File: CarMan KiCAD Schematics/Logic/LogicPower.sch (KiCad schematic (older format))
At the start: 5 parts, among them U4 PYB20-Q24-S5, U7 LT1763CS8-3.3PBF

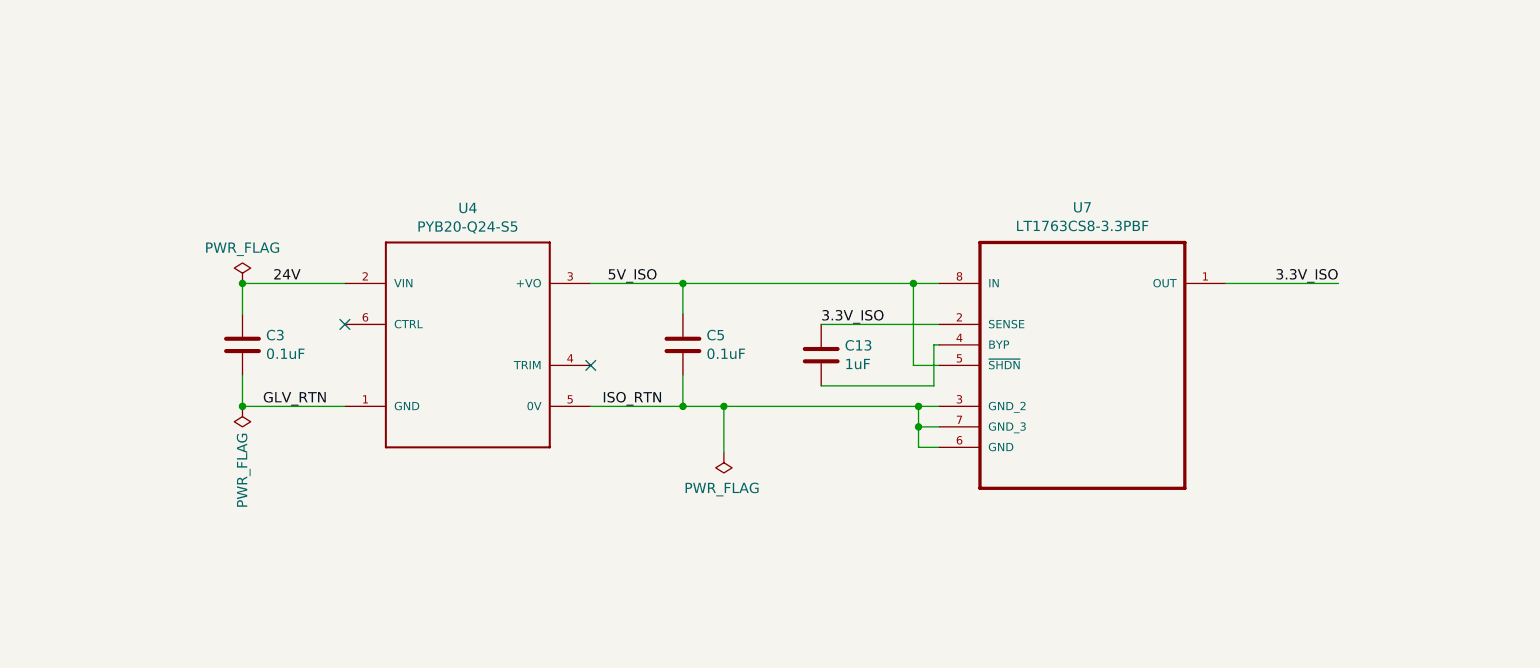
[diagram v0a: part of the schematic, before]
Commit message: Logic Update
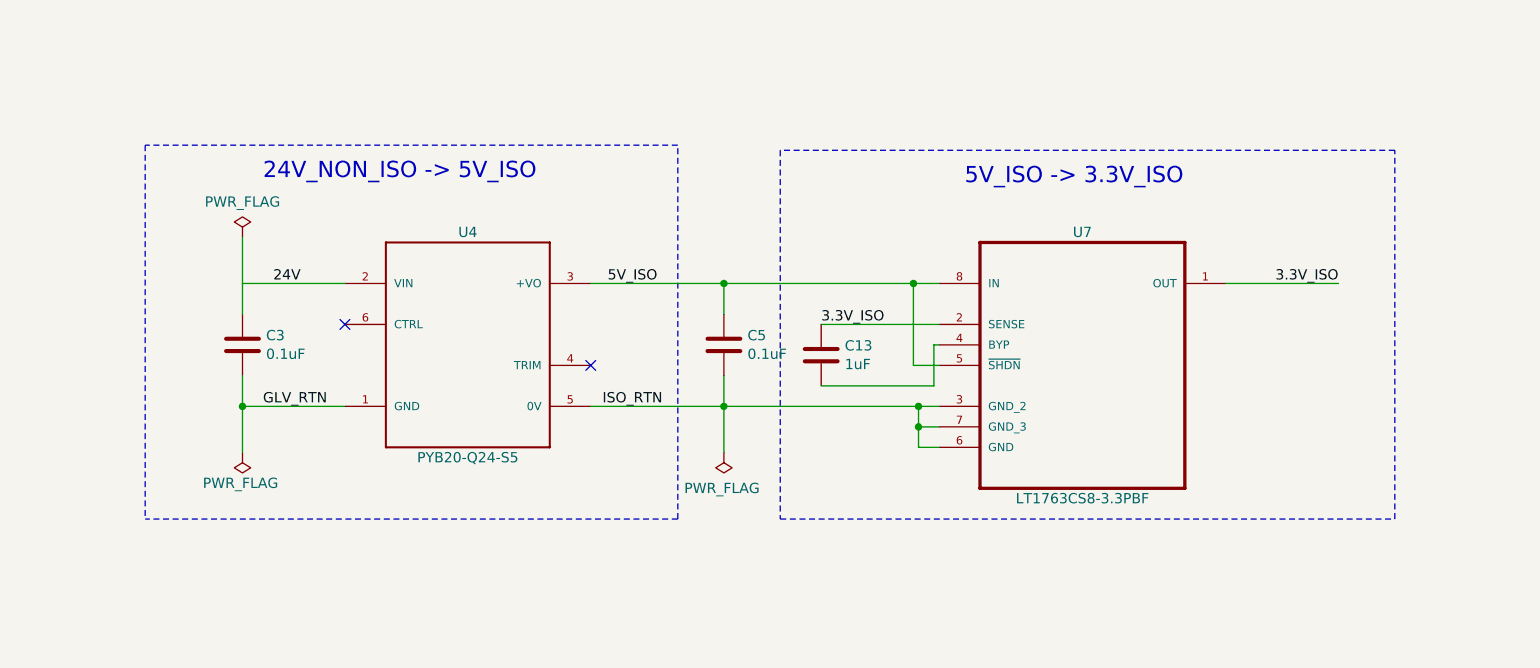
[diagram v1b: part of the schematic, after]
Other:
- note added: "24V_NON_ISO -> 5V_ISO"
- note added: "5V_ISO -> 3.3V_ISO"
- moved on the sheet: C5
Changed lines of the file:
@@
 L Device:C C5
 U 1 1 5FAF6616
-P 5500 3775
-F 0 "C5" H 5615 3821 50  0000 L CNN
-F 1 "0.1uF" H 5615 3730 50  0000 L CNN
-F 2 "Capacitor_SMD:C_0805_2012Metric_Pad1.15x1.40mm_HandSolder" H 5538 3625 50  0001 C CNN
-F 3 "~" H 5500 3775 50  0001 C CNN
-	1    5500 3775
-	1    0    0    -1
-$EndComp
-Wire Wire Line
-	5500 3925 5500 4075
-Wire Wire Line
-	5500 3625 5500 3475
+P 5700 3775
+F 0 "C5" H 5815 3821 50  0000 L CNN
+F 1 "0.1uF" H 5815 3730 50  0000 L CNN
+F 2 "Capacitor_SMD:C_0805_2012Metric_Pad1.15x1.40mm_HandSolder" H 5738 3625 50  0001 C CNN
+F 3 "~" H 5700 3775 50  0001 C CNN
+	1    5700 3775
+	1    0    0    -1
+$EndComp
+Wire Wire Line
+	5700 3925 5700 4075
+Wire Wire Line
+	5700 3625 5700 3475
 $Comp
 L Logic-rescue:C-Device-Logic-rescue C13
@@
 Text Label 5400 4075 2    50   ~ 0
 ISO_RTN
-Wire Wire Line
-	5500 3475 5050 3475
-Connection ~ 5500 3475
-Wire Wire Line
-	5500 4075 5050 4075
-Connection ~ 5500 4075
 $Comp
 L power:PWR_FLAG #FLG03
@@
 AR Path="/5FAF664A" Ref="U?"  Part="1"
 AR Path="/5FAD1CB8/5FAF664A" Ref="U7"  Part="1"
-F 0 "U7" H 7450 4445 50  0000 C CNN
-F 1 "LT1763CS8-3.3PBF" H 7450 4354 50  0000 C CNN
+F 0 "U7" H 7450 4325 50  0000 C CNN
+F 1 "LT1763CS8-3.3PBF" H 7450 3025 50  0000 C CNN
 F 2 "CarMan General Footprints:LT1763CS8-3-PBF" H 7450 3775 50  0001 L BNN
 F 3 "Voltage stabiliser; LDO, fixed; 3.3V; 500mA; SO8; SMD" H 7450 3775 50  0001 L BNN
@@
 U 1 1 5FAF8405
 P 4450 3775
-F 0 "U4" H 4450 4442 50  0000 C CNN
-F 1 "PYB20-Q24-S5" H 4450 4351 50  0000 C CNN
+F 0 "U4" H 4450 4325 50  0000 C CNN
+F 1 "PYB20-Q24-S5" H 4450 3225 50  0000 C CNN
 F 2 "CarMan General Footprints:CONV_PYB20-Q24-S5" H 4450 3775 50  0001 L BNN
 F 3 "CUI Inc" H 4450 3775 50  0001 L BNN
@@
 	3350 3475 3350 3625
 Wire Wire Line
-	3350 3925 3350 4075
-Wire Wire Line
 	3350 4075 3850 4075
 Text Label 3450 4075 0    50   ~ 0
@@
 L power:PWR_FLAG #FLG01
 U 1 1 5FAFECF7
-P 3350 3475
-F 0 "#FLG01" H 3350 3550 50  0001 C CNN
-F 1 "PWR_FLAG" H 3350 3648 50  0000 C CNN
-F 2 "" H 3350 3475 50  0001 C CNN
-F 3 "~" H 3350 3475 50  0001 C CNN
-	1    3350 3475
-	1    0    0    -1
-$EndComp
-Connection ~ 3350 3475
+P 3350 3250
+F 0 "#FLG01" H 3350 3325 50  0001 C CNN
+F 1 "PWR_FLAG" H 3350 3423 50  0000 C CNN
+F 2 "" H 3350 3250 50  0001 C CNN
+F 3 "~" H 3350 3250 50  0001 C CNN
+	1    3350 3250
+	1    0    0    -1
+$EndComp
 $Comp
 L power:PWR_FLAG #FLG0101
 U 1 1 5FB6EF51
-P 3350 4075
-F 0 "#FLG0101" H 3350 4150 50  0001 C CNN
-F 1 "PWR_FLAG" V 3350 4203 50  0000 L CNN
-F 2 "" H 3350 4075 50  0001 C CNN
-F 3 "~" H 3350 4075 50  0001 C CNN
-	1    3350 4075
+P 3350 4300
+F 0 "#FLG0101" H 3350 4375 50  0001 C CNN
+F 1 "PWR_FLAG" H 3175 4450 50  0000 L CNN
+F 2 "" H 3350 4300 50  0001 C CNN
+F 3 "~" H 3350 4300 50  0001 C CNN
+	1    3350 4300
 	-1   0    0    1
 $EndComp
-Connection ~ 3350 4075
-Wire Wire Line
-	5500 4075 5700 4075
 Wire Wire Line
 	5700 4075 5700 4300
@@
 3.3V_ISO
 Wire Wire Line
-	5500 3475 6625 3475
-Wire Wire Line
 	6625 3475 6625 3875
 Connection ~ 6625 3475
@@
 Text Notes 7125 6925 0    185  ~ 0
 24V -> 5V_ISO & 3.3V_ISO
+Wire Notes Line
+	5975 4625 8975 4625
+Wire Notes Line
+	8975 4625 8975 2825
+Wire Notes Line
+	8975 2825 5975 2825
+Wire Notes Line
+	5975 2825 5975 4625
+Text Notes 6875 3000 0    79   ~ 0
+5V_ISO -> 3.3V_ISO
+Connection ~ 5700 3475
+Wire Wire Line
+	5700 3475 6625 3475
+Wire Wire Line
+	5050 3475 5700 3475
+Wire Wire Line
+	5050 4075 5700 4075
+Wire Notes Line
+	5475 4625 5475 2800
+Wire Notes Line
+	5475 2800 2875 2800
+Wire Notes Line
+	5475 4625 2875 4625
+Wire Notes Line
+	2875 2800 2875 4625
+Wire Wire Line
+	3350 4075 3350 4300
+Wire Wire Line
+	3350 3925 3350 4075
+Connection ~ 3350 4075
+Wire Wire Line
+	3350 3250 3350 3475
+Text Notes 3450 2975 0    79   ~ 0
+24V_NON_ISO -> 5V_ISO
 $EndSCHEMATC
